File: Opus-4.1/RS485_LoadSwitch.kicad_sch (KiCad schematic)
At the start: 10 parts, among them J1 PWR_IN, J2 RS485, J3 OUT1, J4 OUT2, J5 OUT3, J6 OUT4, J7 SWD

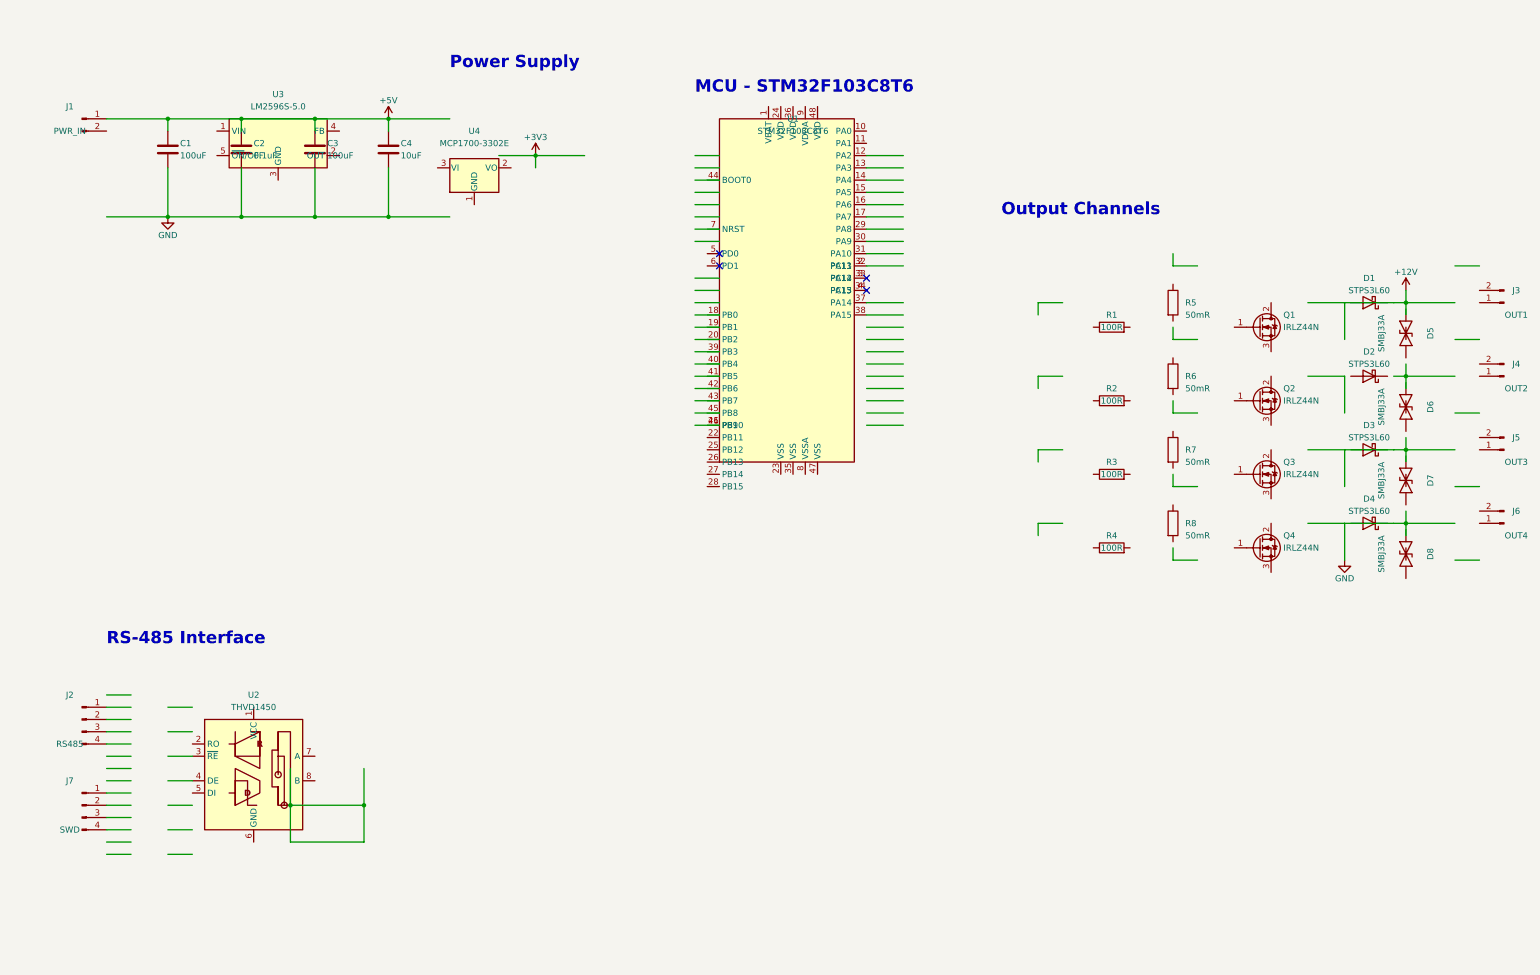
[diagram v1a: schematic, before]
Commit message: Add files via upload
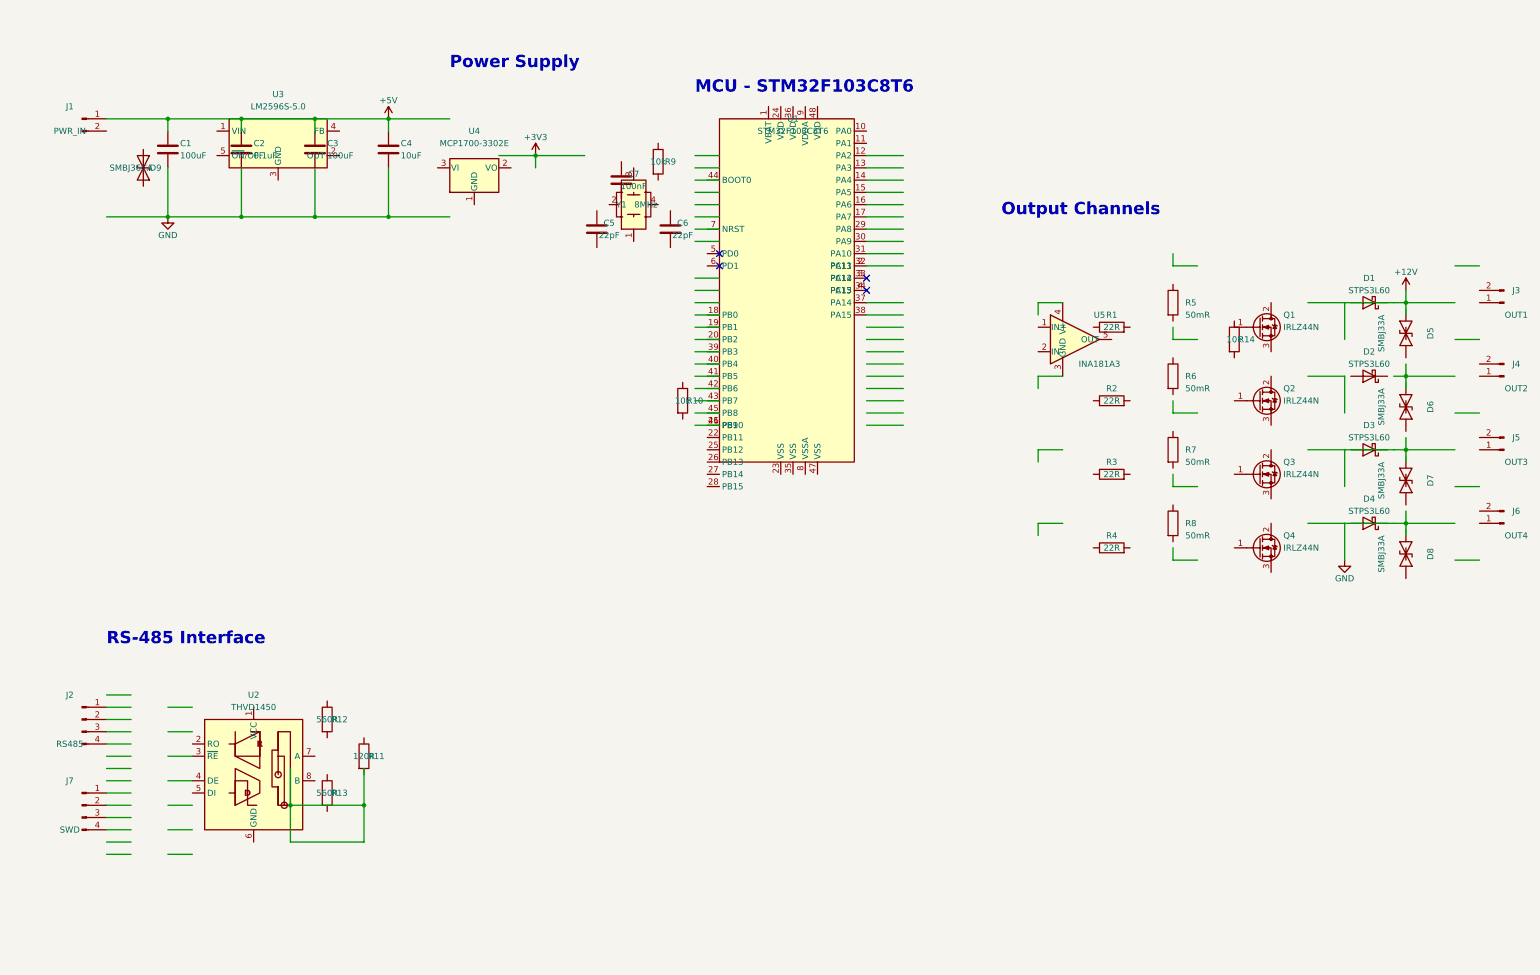
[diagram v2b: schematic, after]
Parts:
- added C5, C6: 22pF, Capacitor_SMD:C_0603_1608Metric, symbol Device:C
- added C7: 100nF, Capacitor_SMD:C_0603_1608Metric, symbol Device:C
- added D9: SMBJ36CA, Diode_SMD:D_SMB, symbol Device:D_TVS
- added R10, R14, R9: 10k, Resistor_SMD:R_0603_1608Metric, symbol Device:R
- added R11: 120R, Resistor_SMD:R_0805_2012Metric, symbol Device:R
- added R12, R13: 560R, Resistor_SMD:R_0603_1608Metric, symbol Device:R
- added U5: INA181A3, Package_TO_SOT_SMD:SOT-23-5, symbol Amplifier_Current:INA181
- added Y1: 8MHz, Crystal:Crystal_SMD_HC49-SD, symbol Device:Crystal_GND24
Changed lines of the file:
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@@
     (comment 4 "STM32F103C8T6 Based Controller")
+  )
+  (symbol (lib_id "Device:Crystal_GND24") (at 147.32 68.58 90) (unit 1)
+    (in_bom yes) (on_board yes) (dnp no)
+    (uuid XTAL1)
+    (property "Reference" "Y1" (at 144.78 68.58 90))
+    (property "Value" "8MHz" (at 149.86 68.58 90))
+    (property "Footprint" "Crystal:Crystal_SMD_HC49-SD" (at 147.32 68.58 0)
+      (effects (font (size 1.27 1.27)) hide))
+    (pin "1" (uuid XTAL1-1))
+    (pin "2" (uuid XTAL1-2))
+    (pin "3" (uuid XTAL1-3))
+    (pin "4" (uuid XTAL1-4))
+  )
+  (symbol (lib_id "Device:C") (at 139.7 73.66 0) (unit 1)
+    (in_bom yes) (on_board yes) (dnp no)
+    (uuid C_OSC1)
+    (property "Reference" "C5" (at 142.24 72.39 0))
+    (property "Value" "22pF" (at 142.24 74.93 0))
+    (property "Footprint" "Capacitor_SMD:C_0603_1608Metric" (at 140.6652 77.47 0)
+      (effects (font (size 1.27 1.27)) hide))
+    (pin "1" (uuid C_OSC1-1))
+    (pin "2" (uuid C_OSC1-2))
+  )
+  (symbol (lib_id "Device:C") (at 154.94 73.66 0) (unit 1)
+    (in_bom yes) (on_board yes) (dnp no)
+    (uuid C_OSC2)
+    (property "Reference" "C6" (at 157.48 72.39 0))
+    (property "Value" "22pF" (at 157.48 74.93 0))
+    (property "Footprint" "Capacitor_SMD:C_0603_1608Metric" (at 155.9052 77.47 0)
+      (effects (font (size 1.27 1.27)) hide))
+    (pin "1" (uuid C_OSC2-1))
+    (pin "2" (uuid C_OSC2-2))
+  )
+  (symbol (lib_id "Device:R") (at 152.4 59.69 0) (unit 1)
+    (in_bom yes) (on_board yes) (dnp no)
+    (uuid R_RST)
+    (property "Reference" "R9" (at 154.94 59.69 0))
+    (property "Value" "10k" (at 152.4 59.69 0))
+    (property "Footprint" "Resistor_SMD:R_0603_1608Metric" (at 150.622 59.69 90)
+      (effects (font (size 1.27 1.27)) hide))
+    (pin "1" (uuid R_RST-1))
+    (pin "2" (uuid R_RST-2))
+  )
+  (symbol (lib_id "Device:C") (at 144.78 63.5 0) (unit 1)
+    (in_bom yes) (on_board yes) (dnp no)
+    (uuid C_RST)
+    (property "Reference" "C7" (at 147.32 62.23 0))
+    (property "Value" "100nF" (at 147.32 64.77 0))
+    (property "Footprint" "Capacitor_SMD:C_0603_1608Metric" (at 145.7452 67.31 0)
+      (effects (font (size 1.27 1.27)) hide))
+    (pin "1" (uuid C_RST-1))
+    (pin "2" (uuid C_RST-2))
+  )
+  (symbol (lib_id "Device:R") (at 157.48 109.22 0) (unit 1)
+    (in_bom yes) (on_board yes) (dnp no)
+    (uuid R_BOOT0)
+    (property "Reference" "R10" (at 160.02 109.22 0))
+    (property "Value" "10k" (at 157.48 109.22 0))
+    (property "Footprint" "Resistor_SMD:R_0603_1608Metric" (at 155.702 109.22 90)
+      (effects (font (size 1.27 1.27)) hide))
+    (pin "1" (uuid R_BOOT0-1))
+    (pin "2" (uuid R_BOOT0-2))
+  )
+  (symbol (lib_id "Amplifier_Current:INA181") (at 238.76 96.52 0) (unit 1)
+    (in_bom yes) (on_board yes) (dnp no)
+    (uuid INA1)
+    (property "Reference" "U5" (at 243.84 91.44 0))
+    (property "Value" "INA181A3" (at 243.84 101.6 0))
+    (property "Footprint" "Package_TO_SOT_SMD:SOT-23-5" (at 238.76 96.52 0)
+      (effects (font (size 1.27 1.27)) hide))
+    (pin "1" (uuid INA1-1))
+    (pin "2" (uuid INA1-2))
+    (pin "3" (uuid INA1-3))
+    (pin "4" (uuid INA1-4))
+    (pin "5" (uuid INA1-5))
+  )
+  (symbol (lib_id "Device:R") (at 91.44 182.88 0) (unit 1)
+    (in_bom yes) (on_board yes) (dnp no)
+    (uuid R_TERM)
+    (property "Reference" "R11" (at 93.98 182.88 0))
+    (property "Value" "120R" (at 91.44 182.88 0))
+    (property "Footprint" "Resistor_SMD:R_0805_2012Metric" (at 89.662 182.88 90)
+      (effects (font (size 1.27 1.27)) hide))
+    (pin "1" (uuid R_TERM-1))
+    (pin "2" (uuid R_TERM-2))
+  )
+  (symbol (lib_id "Device:R") (at 83.82 175.26 0) (unit 1)
+    (in_bom yes) (on_board yes) (dnp no)
+    (uuid R_BIAS_UP)
+    (property "Reference" "R12" (at 86.36 175.26 0))
+    (property "Value" "560R" (at 83.82 175.26 0))
+    (property "Footprint" "Resistor_SMD:R_0603_1608Metric" (at 82.042 175.26 90)
+      (effects (font (size 1.27 1.27)) hide))
+    (pin "1" (uuid R_BIAS_UP-1))
+    (pin "2" (uuid R_BIAS_UP-2))
+  )
+  (symbol (lib_id "Device:R") (at 83.82 190.5 0) (unit 1)
+    (in_bom yes) (on_board yes) (dnp no)
+    (uuid R_BIAS_DN)
+    (property "Reference" "R13" (at 86.36 190.5 0))
+    (property "Value" "560R" (at 83.82 190.5 0))
+    (property "Footprint" "Resistor_SMD:R_0603_1608Metric" (at 82.042 190.5 90)
+      (effects (font (size 1.27 1.27)) hide))
+    (pin "1" (uuid R_BIAS_DN-1))
+    (pin "2" (uuid R_BIAS_DN-2))
   )
   (junction (at 50.8 50.8) (diameter 0) (color 0 0 0 0)
@@
       (effects (font (size 1.27 1.27)))
     )
-    (property "Value" "100R" (at 246.38 93.98 90)
+    (property "Value" "22R" (at 246.38 93.98 90)
       (effects (font (size 1.27 1.27)))
     )
@@
       (effects (font (size 1.27 1.27)))
     )
-    (property "Value" "100R" (at 246.38 109.22 90)
+    (property "Value" "22R" (at 246.38 109.22 90)
       (effects (font (size 1.27 1.27)))
     )
@@
       (effects (font (size 1.27 1.27)))
     )
-    (property "Value" "100R" (at 246.38 124.46 90)
+    (property "Value" "22R" (at 246.38 124.46 90)
       (effects (font (size 1.27 1.27)))
     )
@@
       (effects (font (size 1.27 1.27)))
     )
-    (property "Value" "100R" (at 246.38 139.7 90)
+    (property "Value" "22R" (at 246.38 139.7 90)
       (effects (font (size 1.27 1.27)))
     )
@@
     )
   )
+  (symbol (lib_id "Device:R") (at 271.78 96.52 0) (unit 1)
+    (in_bom yes) (on_board yes) (dnp no)
+    (uuid R_GATE_PD1)
+    (property "Reference" "R14" (at 274.32 96.52 0))
+    (property "Value" "10k" (at 271.78 96.52 0))
+    (property "Footprint" "Resistor_SMD:R_0603_1608Metric" (at 270.002 96.52 90)
+      (effects (font (size 1.27 1.27)) hide))
+    (pin "1" (uuid R_GATE_PD1-1))
+    (pin "2" (uuid R_GATE_PD1-2))
+  )
+  (symbol (lib_id "Device:D_TVS") (at 45.72 60.96 270) (unit 1)
+    (in_bom yes) (on_board yes) (dnp no)
+    (uuid TVS_IN)
+    (property "Reference" "D9" (at 48.26 60.96 90))
+    (property "Value" "SMBJ36CA" (at 43.18 60.96 90))
+    (property "Footprint" "Diode_SMD:D_SMB" (at 45.72 60.96 0)
+      (effects (font (size 1.27 1.27)) hide))
+    (pin "1" (uuid TVS_IN-1))
+    (pin "2" (uuid TVS_IN-2))
+  )
   (symbol (lib_id "Device:R") (at 259.08 88.9 0) (unit 1)

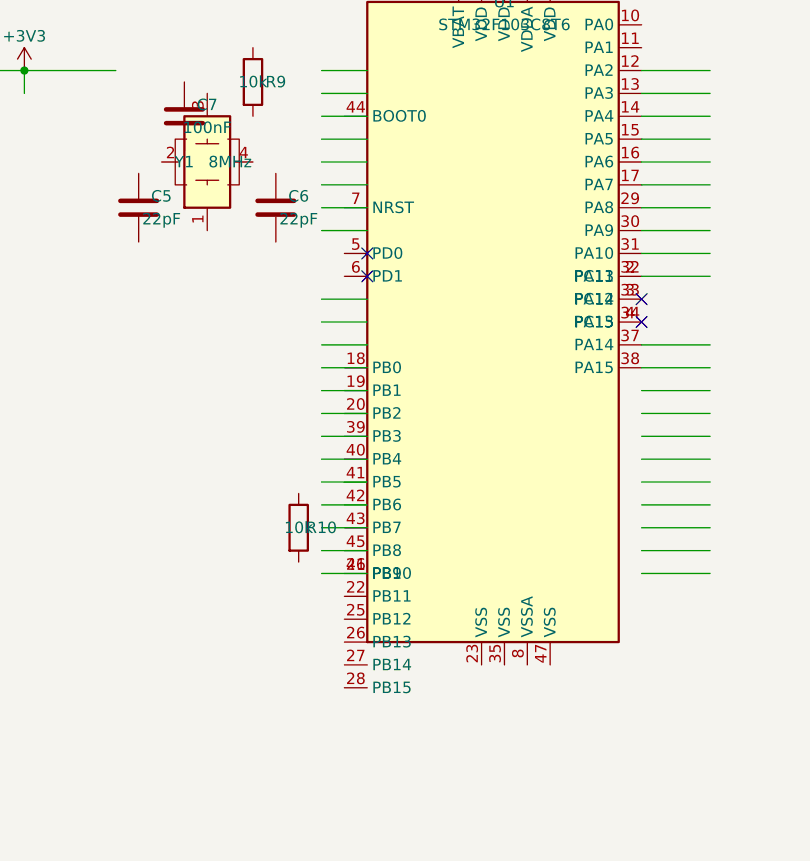
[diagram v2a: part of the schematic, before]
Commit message: Add files via upload
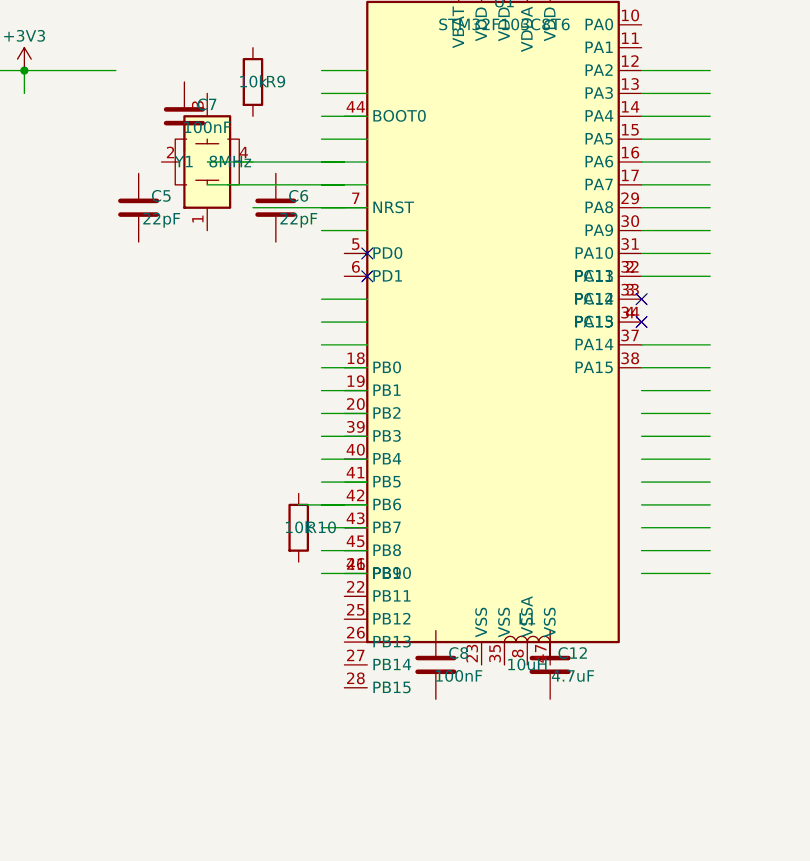
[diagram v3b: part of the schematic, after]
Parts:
- added C12: 4.7uF, Capacitor_SMD:C_0805_2012Metric, symbol Device:C
- added C8: 100nF, Capacitor_SMD:C_0603_1608Metric, symbol Device:C
- added L1: 10uH, Inductor_SMD:L_0805_2012Metric, symbol Device:L
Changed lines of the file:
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@@
     )
+  )
+  (wire (pts (xy 162.56 68.58) (xy 147.32 68.58))
+    (stroke (width 0) (type default))
+    (uuid W_XTAL1))
+  (wire (pts (xy 162.56 71.12) (xy 147.32 71.12))
+    (stroke (width 0) (type default))
+    (uuid W_XTAL2))
+  (wire (pts (xy 162.56 73.66) (xy 152.4 73.66))
+    (stroke (width 0) (type default))
+    (uuid W_RST))
+  (wire (pts (xy 162.56 106.68) (xy 157.48 106.68))
+    (stroke (width 0) (type default))
+    (uuid W_BOOT0))
+  (symbol (lib_id "Device:C") (at 172.72 124.46 0) (unit 1)
+    (in_bom yes) (on_board yes) (dnp no)
+    (uuid C_VDD1)
+    (property "Reference" "C8" (at 175.26 123.19 0))
+    (property "Value" "100nF" (at 175.26 125.73 0))
+    (property "Footprint" "Capacitor_SMD:C_0603_1608Metric" (at 173.6852 128.27 0)
+      (effects (font (size 1.27 1.27)) hide))
+  )
+  (symbol (lib_id "Device:C") (at 185.42 124.46 0) (unit 1)
+    (in_bom yes) (on_board yes) (dnp no)
+    (uuid C_VDDA)
+    (property "Reference" "C12" (at 187.96 123.19 0))
+    (property "Value" "4.7uF" (at 187.96 125.73 0))
+    (property "Footprint" "Capacitor_SMD:C_0805_2012Metric" (at 186.3852 128.27 0)
+      (effects (font (size 1.27 1.27)) hide))
+  )
+  (symbol (lib_id "Device:L") (at 182.88 121.92 90) (unit 1)
+    (in_bom yes) (on_board yes) (dnp no)
+    (uuid L_VDDA)
+    (property "Reference" "L1" (at 182.88 119.38 90))
+    (property "Value" "10uH" (at 182.88 124.46 90))
+    (property "Footprint" "Inductor_SMD:L_0805_2012Metric" (at 182.88 121.92 0)
+      (effects (font (size 1.27 1.27)) hide))
   )
   (symbol (lib_id "Interface_UART:THVD1450") (at 68.58 185.42 0) (unit 1)

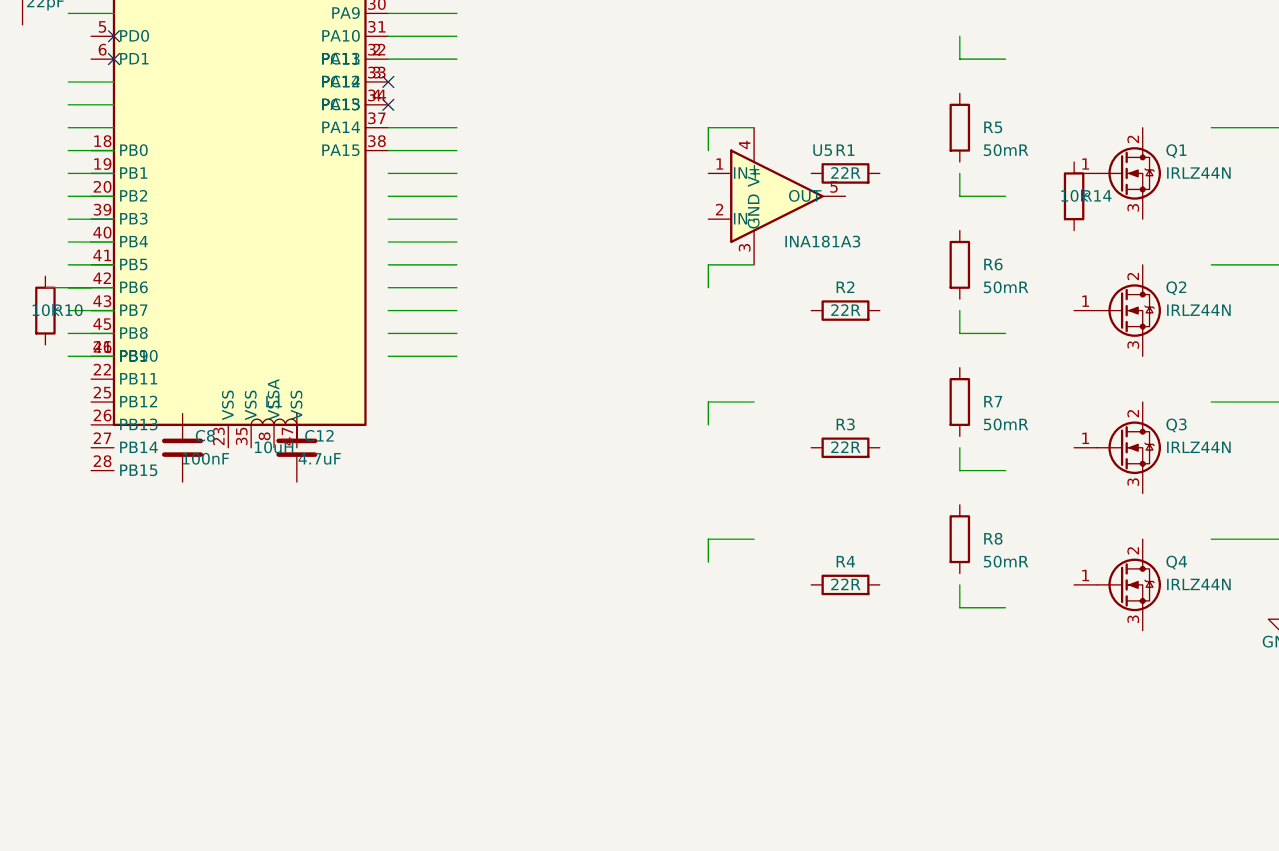
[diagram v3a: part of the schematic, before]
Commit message: Add files via upload
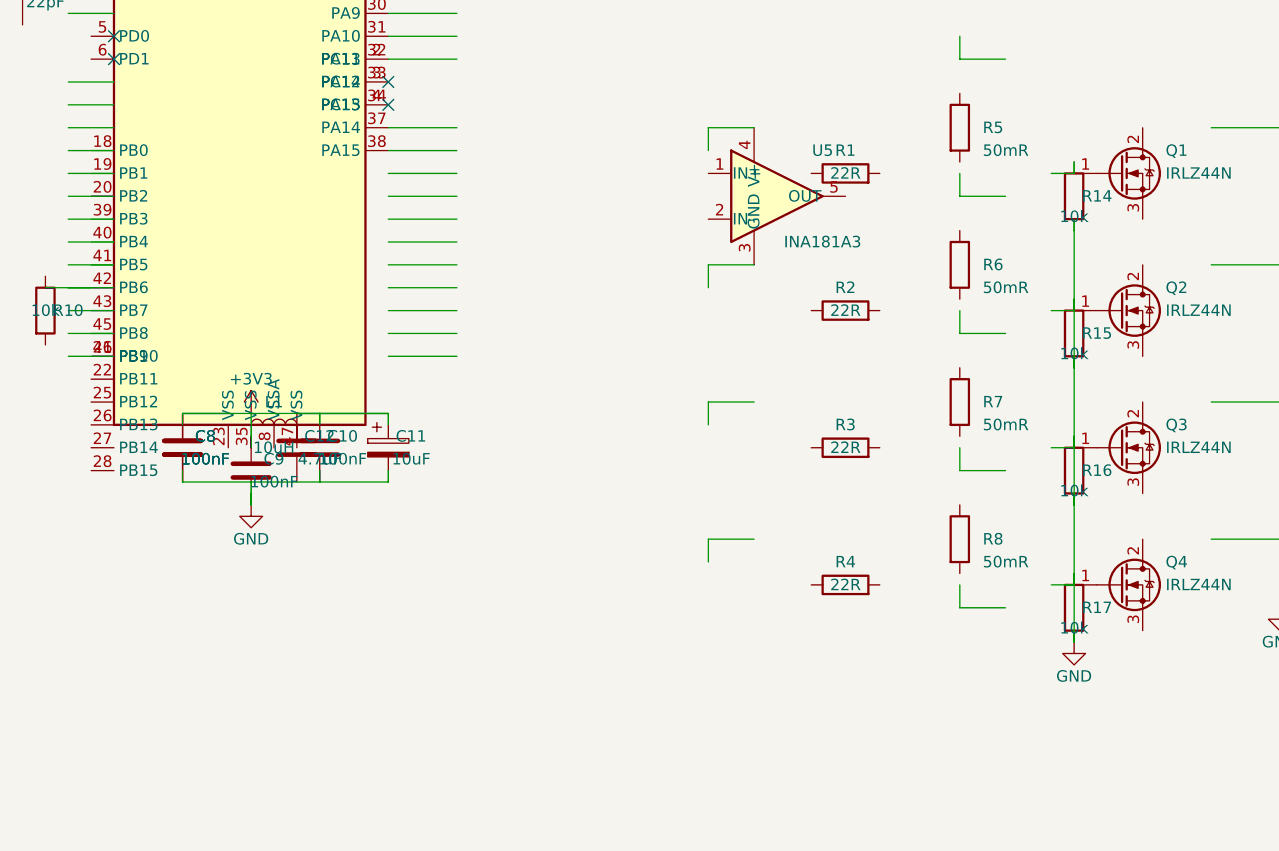
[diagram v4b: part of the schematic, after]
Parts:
- added C10, C8, C9: 100nF, Capacitor_SMD:C_0603_1608Metric, symbol Device:C
- added C11: 10uF, Capacitor_SMD:CP_Elec_5x5.4, symbol Device:CP
- added R15, R16, R17: 10k, Resistor_SMD:R_0603_1608Metric, symbol Device:R
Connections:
- net +3V3: now also C12.1, C8.1, J3.35 (VSS), C10.1, C11.1, C8.1, C9.1
- net GND: now also C8.2, D6.1 (A1), D7.1 (A1), D8.1 (A1), R14.2, C10.2, C11.2, C8.2, C9.2, R15.1, R15.2, R16.1, R16.2, R17.1, R17.2
- net at J7.1 (Pin_1): now also R14.1
